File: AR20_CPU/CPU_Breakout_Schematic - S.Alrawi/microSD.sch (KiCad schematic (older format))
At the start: 6 parts, among them U1 74LCX125M, U2 MCP1700_SOT23

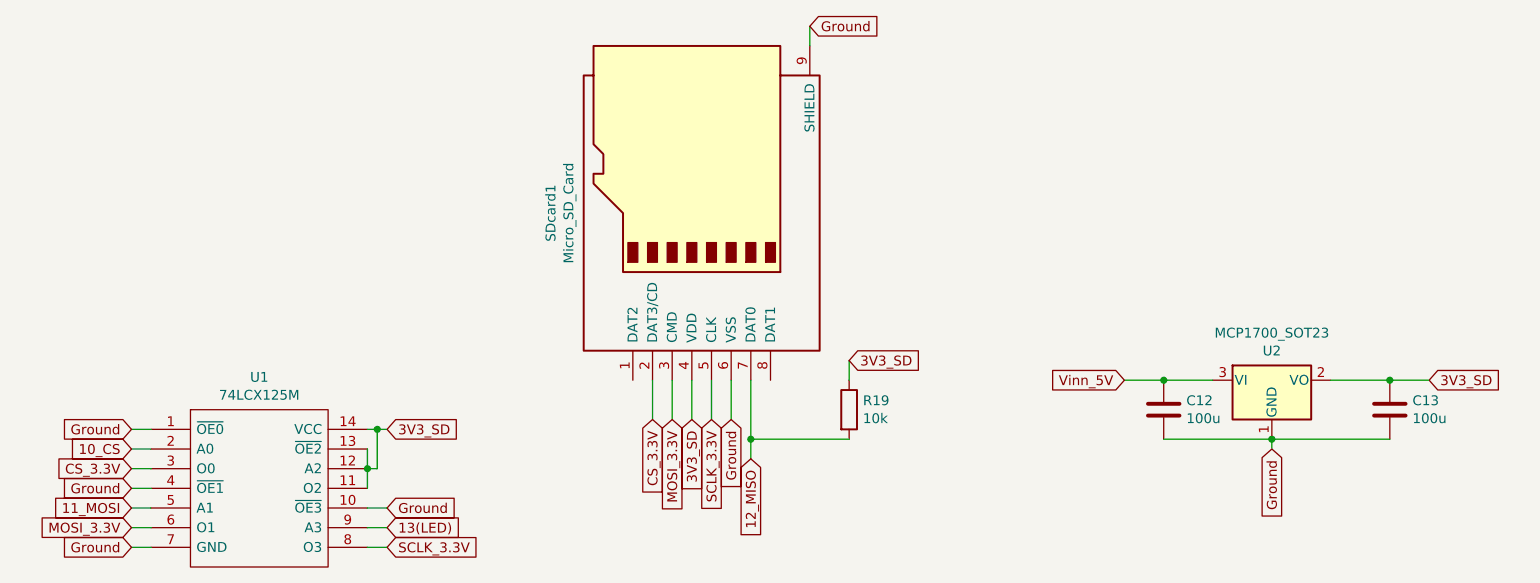
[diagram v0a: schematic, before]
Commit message: BreakoutBoard final edit
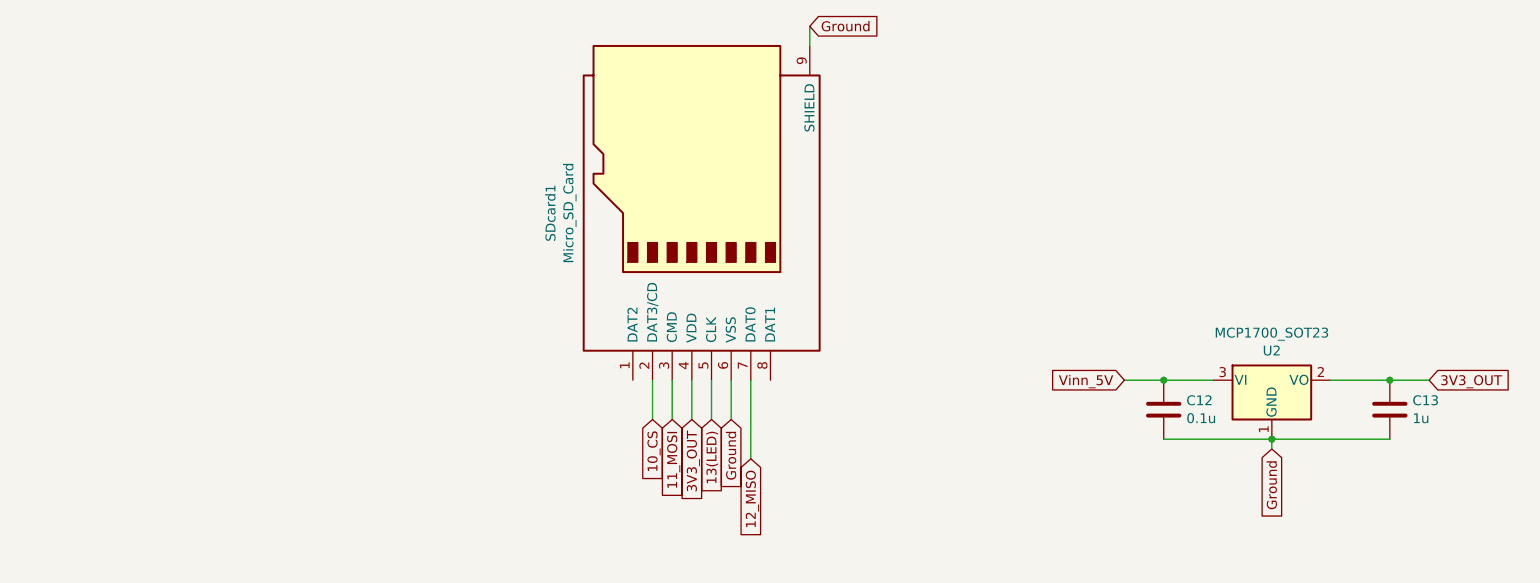
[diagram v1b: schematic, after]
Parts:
- removed R18: 10k, Resistor_SMD:R_0603_1608Metric, symbol Device:R
- removed U1: 74LCX125M, SOIC127P600X175-14N, symbol SamacSys_Parts:74LCX125M
- C12: value 100u -> 0.1u
- C13: value 100u -> 1u
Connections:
- net CS_3.3V is gone; now on net 10_CS: SDcard1.2 (DAT3/CD)
- net MOSI_3.3V is gone; now on net 11_MOSI: SDcard1.3 (CMD)
- net SCLK_3.3V is gone; now on net 13(LED): SDcard1.5 (CLK)
- net 3V3_SD renamed 3V3_OUT
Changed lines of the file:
@@
 	1    0    0    -1
 $EndComp
-Text GLabel 9100 3500 2    50   Input ~ 0
-3V3_SD
-Wire Wire Line
-	6150 3400 6150 3500
 Wire Wire Line
 	5950 1800 5950 1700
-Text GLabel 5350 3700 3    50   Input ~ 0
-3V3_SD
 Wire Wire Line
 	5250 3700 5250 3500
@@
 Wire Wire Line
 	5350 3700 5350 3500
-Wire Wire Line
-	5150 3700 5150 3500
-Text GLabel 3800 4250 2    50   Input ~ 0
-13(LED)
-Text GLabel 2500 3850 0    50   Input ~ 0
-10_CS
-Text GLabel 2500 4150 0    50   Input ~ 0
-11_MOSI
 Text GLabel 5650 3900 3    50   Input ~ 0
 12_MISO
+Text GLabel 5550 3700 3    50   Input ~ 0
+Ground
+Text GLabel 5950 1700 2    50   Input ~ 0
+Ground
+Wire Wire Line
+	7750 3800 8300 3800
+Connection ~ 8300 3800
+Wire Wire Line
+	8300 3800 8900 3800
+Wire Wire Line
+	7550 3500 7750 3500
+Wire Wire Line
+	8000 3500 7750 3500
+Connection ~ 7750 3500
+$Comp
+L Device:C C12
+U 1 1 5DE5A450
+P 7750 3650
+F 0 "C12" H 7635 3604 50  0000 R CNN
+F 1 "0.1u" H 7635 3695 50  0000 R CNN
+F 2 "Capacitor_SMD:C_0603_1608Metric" H 7788 3500 50  0001 C CNN
+F 3 "~" H 7750 3650 50  0001 C CNN
+	1    7750 3650
+	-1   0    0    1
+$EndComp
+Text GLabel 9100 3500 2    50   Input ~ 0
+3V3_OUT
+Wire Wire Line
+	8900 3500 8600 3500
+Wire Wire Line
+	9100 3500 8900 3500
+Connection ~ 8900 3500
+$Comp
+L Device:C C13
+U 1 1 5DE59DD0
+P 8900 3650
+F 0 "C13" H 8785 3604 50  0000 R CNN
+F 1 "1u" H 8785 3695 50  0000 R CNN
+F 2 "Capacitor_SMD:C_0603_1608Metric" H 8938 3500 50  0001 C CNN
+F 3 "~" H 8900 3650 50  0001 C CNN
+	1    8900 3650
+	-1   0    0    1
+$EndComp
+Text GLabel 5150 3700 3    50   Input ~ 0
+10_CS
+Text GLabel 5450 3700 3    50   Input ~ 0
+13(LED)
+Text GLabel 5250 3700 3    50   Input ~ 0
+11_MOSI
+Text GLabel 5350 3700 3    50   Input ~ 0
+3V3_OUT
+Wire Wire Line
+	5650 3500 5650 3900
 $Comp
 L Connector:Micro_SD_Card SDcard?
@@
 	0    -1   -1   0
 $EndComp
-Text GLabel 5550 3700 3    50   Input ~ 0
-Ground
-Text GLabel 5950 1700 2    50   Input ~ 0
-Ground
-Text GLabel 5150 3700 3    50   Input ~ 0
-CS_3.3V
-Text GLabel 2500 3950 0    50   Input ~ 0
-CS_3.3V
-Text GLabel 5250 3700 3    50   Input ~ 0
-MOSI_3.3V
-Text GLabel 2500 4250 0    50   Input ~ 0
-MOSI_3.3V
-Text GLabel 2500 4350 0    50   Input ~ 0
-Ground
-Text GLabel 5450 3700 3    50   Input ~ 0
-SCLK_3.3V
-Text GLabel 3800 4350 2    50   Input ~ 0
-SCLK_3.3V
-Text GLabel 3800 3750 2    50   Input ~ 0
-3V3_SD
-Text GLabel 2500 3750 0    50   Input ~ 0
-Ground
-Text GLabel 3800 4150 2    50   Input ~ 0
-Ground
 Wire Wire Line
-	3800 4350 3700 4350
-Wire Wire Line
-	3800 4250 3700 4250
-Wire Wire Line
-	3800 4150 3700 4150
-Wire Wire Line
-	2500 3750 2600 3750
-Wire Wire Line
-	2500 3850 2600 3850
-Wire Wire Line
-	2500 3950 2600 3950
-Wire Wire Line
-	2500 4150 2600 4150
-Wire Wire Line
-	2500 4250 2600 4250
-Wire Wire Line
-	2500 4350 2600 4350
-Text GLabel 2500 4050 0    50   Input ~ 0
-Ground
-Wire Wire Line
-	2600 4050 2500 4050
-Text GLabel 6150 3400 2    50   Input ~ 0
-3V3_SD
-Wire Wire Line
-	5650 3500 5650 3800
-Wire Wire Line
-	5650 3800 6150 3800
-Connection ~ 5650 3800
-Wire Wire Line
-	5650 3800 5650 3900
-$Comp
-L SamacSys_Parts:74LCX125M U1
-U 1 1 5DE57AC5
-P 2600 3750
-F 0 "U1" H 3150 4015 50  0000 C CNN
-F 1 "74LCX125M" H 3150 3924 50  0000 C CNN
-F 2 "SOIC127P600X175-14N" H 3550 3850 50  0001 L CNN
-F 3 "https://componentsearchengine.com/Datasheets/1/74LCX125M.pdf" H 3550 3750 50  0001 L CNN
-F 4 "Low Voltage Quad Buffer with 5V Tolerant Inputs and Outputs" H 3550 3650 50  0001 L CNN "Description"
-F 5 "" H 3550 3550 50  0001 L CNN "Height"
-F 6 "512-74LCX125M" H 3550 3450 50  0001 L CNN "Mouser Part Number"
-F 7 "https://www.mouser.com/Search/Refine.aspx?Keyword=512-74LCX125M" H 3550 3350 50  0001 L CNN "Mouser Price/Stock"
-F 8 "ON Semiconductor" H 3550 3250 50  0001 L CNN "Manufacturer_Name"
-F 9 "74LCX125M" H 3550 3150 50  0001 L CNN "Manufacturer_Part_Number"
-	1    2600 3750
-	1    0    0    -1
-$EndComp
-Wire Wire Line
-	3700 3850 3700 3950
-Wire Wire Line
-	3700 4050 3700 3950
-Connection ~ 3700 3950
-Wire Wire Line
-	3700 3750 3750 3750
-Wire Wire Line
-	3750 3750 3750 3950
-Wire Wire Line
-	3750 3950 3700 3950
-Connection ~ 3750 3750
-Wire Wire Line
-	3750 3750 3800 3750
-$Comp
-L Device:C C13
-U 1 1 5DE59DD0
-P 8900 3650
-F 0 "C13" H 8785 3604 50  0000 R CNN
-F 1 "100u" H 8785 3695 50  0000 R CNN
-F 2 "Capacitor_SMD:C_0603_1608Metric" H 8938 3500 50  0001 C CNN
-F 3 "~" H 8900 3650 50  0001 C CNN
-	1    8900 3650
-	-1   0    0    1
-$EndComp
-$Comp
-L Device:C C12
-U 1 1 5DE5A450
-P 7750 3650
-F 0 "C12" H 7635 3604 50  0000 R CNN
-F 1 "100u" H 7635 3695 50  0000 R CNN
-F 2 "Capacitor_SMD:C_0603_1608Metric" H 7788 3500 50  0001 C CNN
-F 3 "~" H 7750 3650 50  0001 C CNN
-	1    7750 3650
-	-1   0    0    1
-$EndComp
-Wire Wire Line
-	9100 3500 8900 3500
-Wire Wire Line
-	8900 3500 8600 3500
-Connection ~ 8900 3500
-Wire Wire Line
-	8000 3500 7750 3500
-Wire Wire Line
-	7550 3500 7750 3500
-Connection ~ 7750 3500
-Wire Wire Line
-	7750 3800 8300 3800
-Connection ~ 8300 3800
-Wire Wire Line
-	8300 3800 8900 3800
-$Comp
-L Device:R R?
-U 1 1 5DFCE3E4
-P 6150 3650
-AR Path="/5DFCE3E4" Ref="R?"  Part="1"
-AR Path="/5DFCB53C/5DFCE3E4" Ref="R18"  Part="1"
-AR Path="/5DE8C4DF/5DFCE3E4" Ref="R19"  Part="1"
-F 0 "R19" H 6220 3696 50  0000 L CNN
-F 1 "10k" H 6220 3605 50  0000 L CNN
-F 2 "Resistor_SMD:R_0603_1608Metric" V 6080 3650 50  0001 C CNN
-F 3 "~" H 6150 3650 50  0001 C CNN
-	1    6150 3650
-	1    0    0    -1
-$EndComp
+	5150 3500 5150 3700
 $EndSCHEMATC
